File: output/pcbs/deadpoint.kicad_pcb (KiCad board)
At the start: 2 copper layers, 113.6 x 118.4 mm, 49 parts

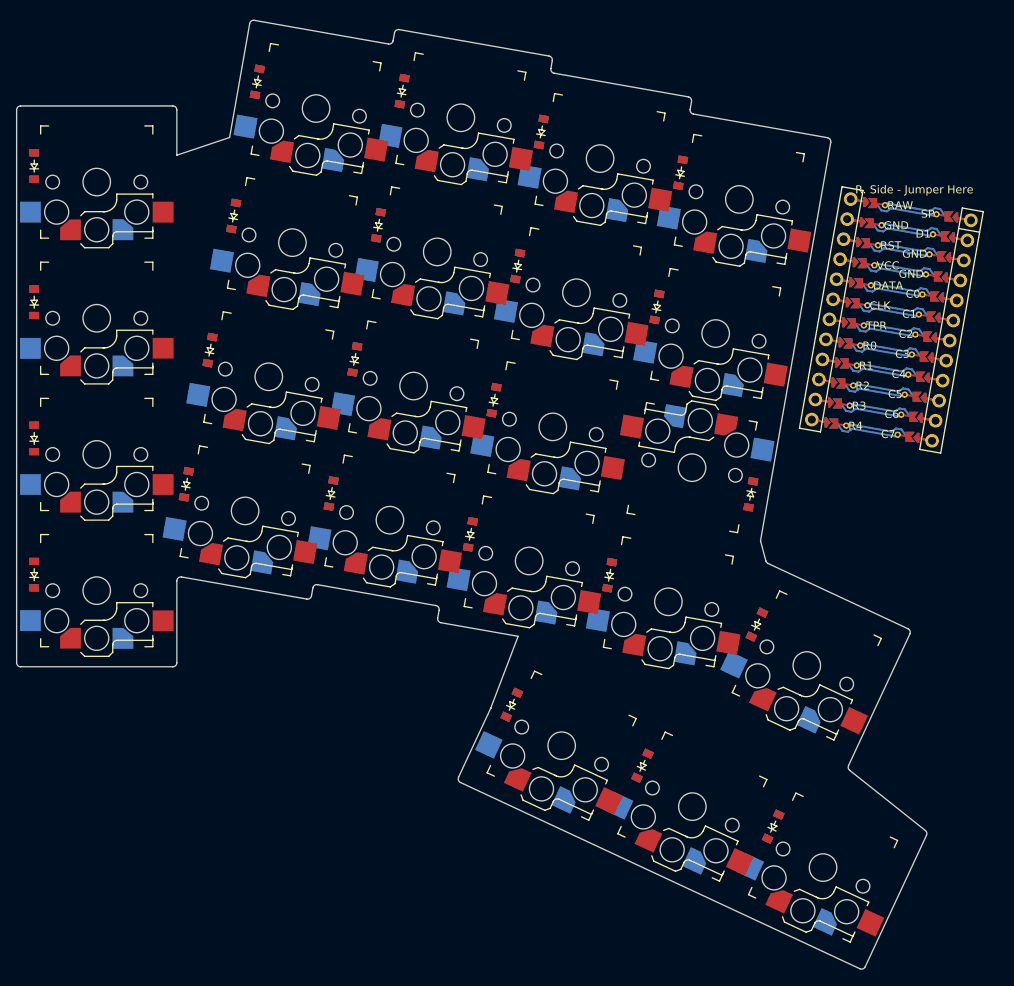
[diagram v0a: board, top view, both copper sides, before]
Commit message: adjust splay
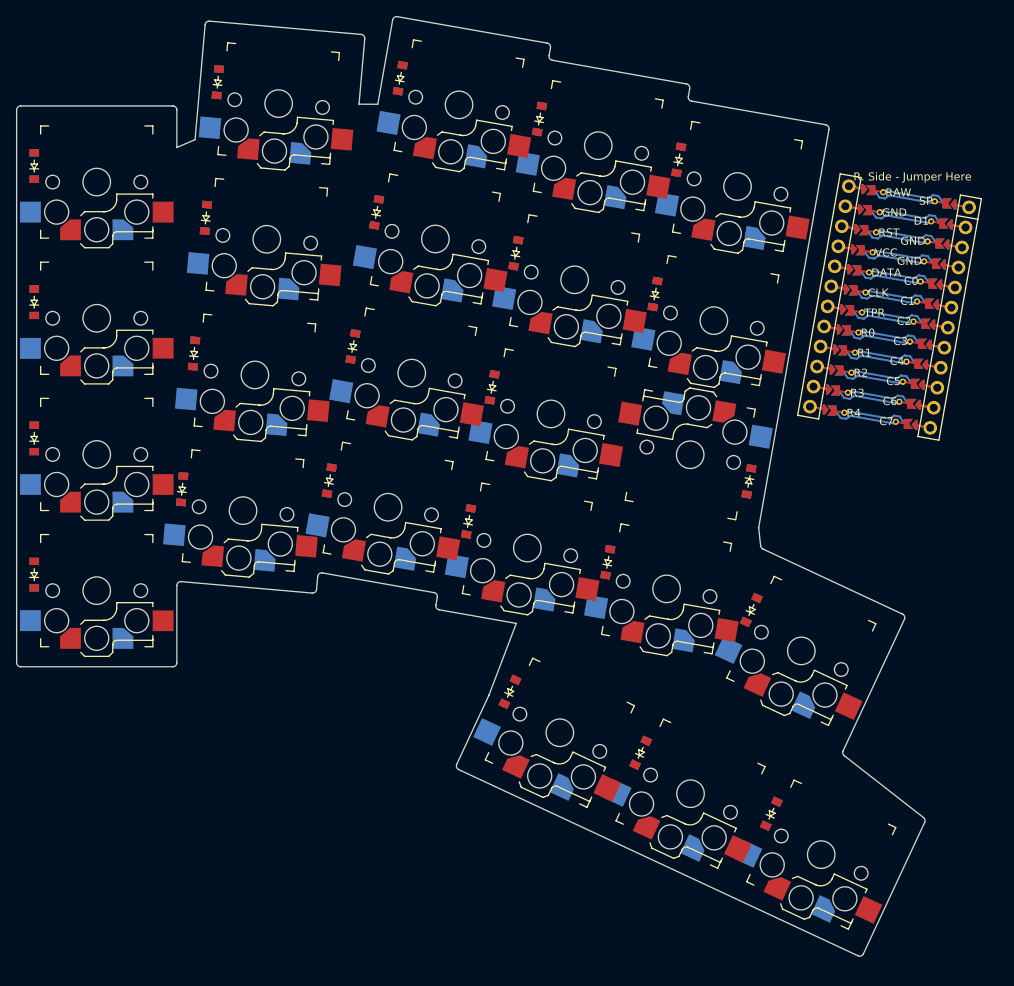
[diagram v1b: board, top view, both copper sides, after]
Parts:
- moved D8 4.93 mm to (115.1, 36.5), turned to 85 degrees
- moved S8 4.71 mm to (122.7, 39.2), turned to 175 degrees
- moved D7 3.47 mm to (113.6, 53.5), turned to 85 degrees
- moved S7 3.23 mm to (121.2, 56.1), turned to 175 degrees
- moved D6 2.04 mm to (112.1, 70.4), turned to 85 degrees
- moved D23 1.95 mm to (181.7, 102.4)
- moved S23 1.95 mm to (187.9, 107.5)
- moved S6 1.74 mm to (119.7, 73.1), turned to 175 degrees
- moved D13 1.63 mm to (146.4, 91.4)
- moved D14 1.63 mm to (149.4, 74.6)
- moved D15 1.63 mm to (152.3, 57.9)
- moved D16 1.63 mm to (155.3, 41.1)
- moved S13 1.63 mm to (153.7, 94.7)
- moved S14 1.63 mm to (156.7, 77.9)
- moved S15 1.63 mm to (159.7, 61.2)
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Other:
- board size 113.6 x 118.4 mm -> 113.4 x 117.3 mm
